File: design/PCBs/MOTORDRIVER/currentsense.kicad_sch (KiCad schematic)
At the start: 0 parts

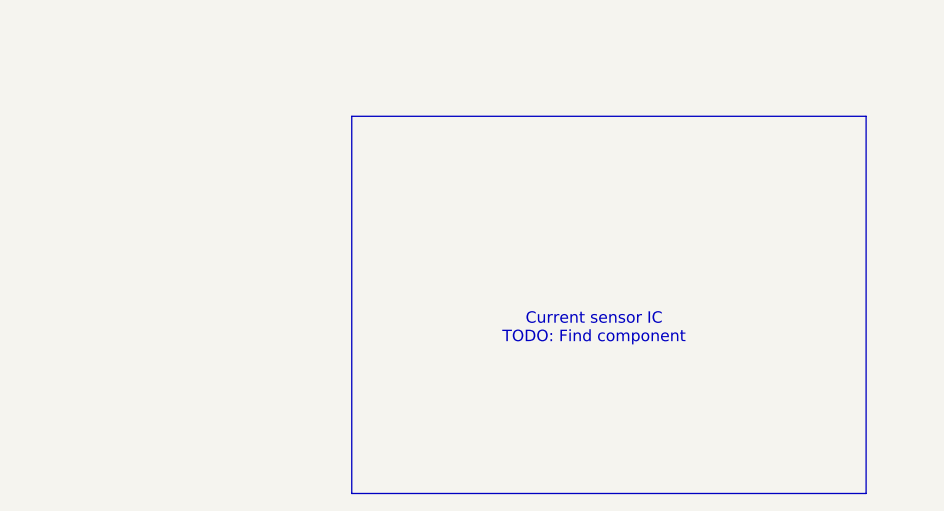
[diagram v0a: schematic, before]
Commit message: updated PCB
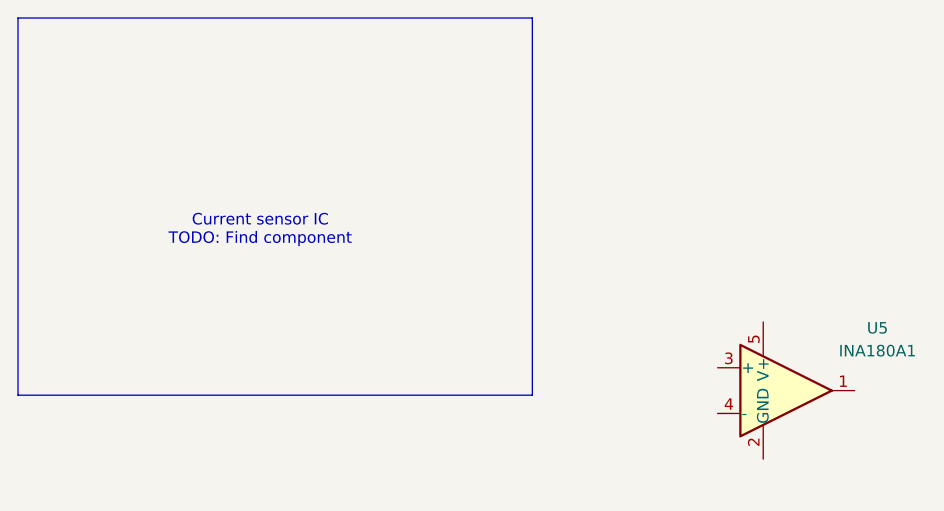
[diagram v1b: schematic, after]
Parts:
- added U5: INA180A1, Package_TO_SOT_SMD:SOT-23-5, symbol Amplifier_Current:INA180A1
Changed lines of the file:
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@@
 	(paper "A4")
 	(rectangle
-		(start 105.41 74.93)
-		(end 162.56 116.84)
+		(start 68.326 64.008)
+		(end 125.476 105.918)
 		(stroke
 			(width 0)
@@
 	(text "Current sensor IC\nTODO: Find component"
 		(exclude_from_sim no)
-		(at 132.334 98.552 0)
+		(at 95.25 87.63 0)
 		(effects
 			(font
@@
 			)
 		)
+	)
+	(symbol
+		(lib_id "Amplifier_Current:INA180A1")
+		(at 153.67 105.41 0)
+		(unit 1)
+		(exclude_from_sim no)
+		(in_bom yes)
+		(on_board yes)
+		(dnp no)
+		(fields_autoplaced yes)
+		(property "Reference" "U5"
+			(at 163.83 98.4755 0)
+			(effects
+				(font
+					(size 1.27 1.27)
+				)
+			)
+		)
+		(property "Value" "INA180A1"
+			(at 163.83 101.0155 0)
+			(effects
+				(font
+					(size 1.27 1.27)
+				)
+			)
+		)
+		(property "Footprint" "Package_TO_SOT_SMD:SOT-23-5"
+			(at 154.94 104.14 0)
+			(effects
+				(font
+					(size 1.27 1.27)
+				)
+				(hide yes)
+			)
+		)
+		(property "Datasheet" "http://www.ti.com/lit/ds/symlink/ina180.pdf"
+			(at 157.48 101.6 0)
+			(effects
+				(font
+					(size 1.27 1.27)
+				)
+				(hide yes)
+			)
+		)
+		(property "Description" "Current Sense Amplifier, 1 Circuit, Rail-to-Rail, 26V, Gain 20 V/V, SOT-23-5"
+			(at 153.67 105.41 0)
+			(effects
+				(font
+					(size 1.27 1.27)
+				)
+				(hide yes)
+			)
+		)
+		(pin "3"
+		)
+		(pin "2"
+		)
+		(pin "1"
+		)
+		(pin "5"
+		)
+		(pin "4"
+		)
+		(instances
+			(project ""
+				(path "/c7634e88-16d1-45ec-9aac-9c841e03cf6d/22c06531-1f6c-46f3-988e-cea008e98016"
+					(reference "U5")
+					(unit 1)
+				)
+				(path "/c7634e88-16d1-45ec-9aac-9c841e03cf6d/474d6285-5514-49ae-8177-1e63fd9cd03e"
+					(reference "U7")
+					(unit 1)
+				)
+				(path "/c7634e88-16d1-45ec-9aac-9c841e03cf6d/721caf15-f1fc-41df-88f3-9bb14360f09a"
+					(reference "U6")
+					(unit 1)
+				)
+			)
+		)
